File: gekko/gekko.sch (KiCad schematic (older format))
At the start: 83 parts, among them J10 Conn_01x02, J11 Conn_01x02, J3 Conn_01x05, J4 Conn_01x03, J6 Conn_01x02, Q5 IRLML6344TRPBFTR, SW1 SW_Push_Dual_x2, SW2 SW_DPDT_x2, U1 DRV8835, U12 sw_pch, U2 STM32F413CH6, U3 LED_FOTR, U4 LP5907_DBV, U5 ICM20648, U6 LED_FOTR, U7 LED_FOTR, U8 LED_FOTR, U9 RP124N334E-TR-FE, Y1 Crystal_GND23

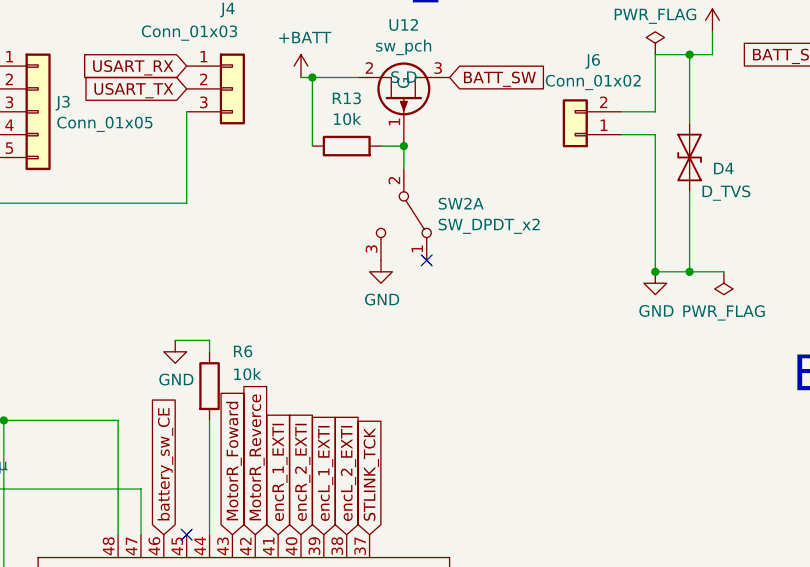
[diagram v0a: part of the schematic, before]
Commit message: betaGND
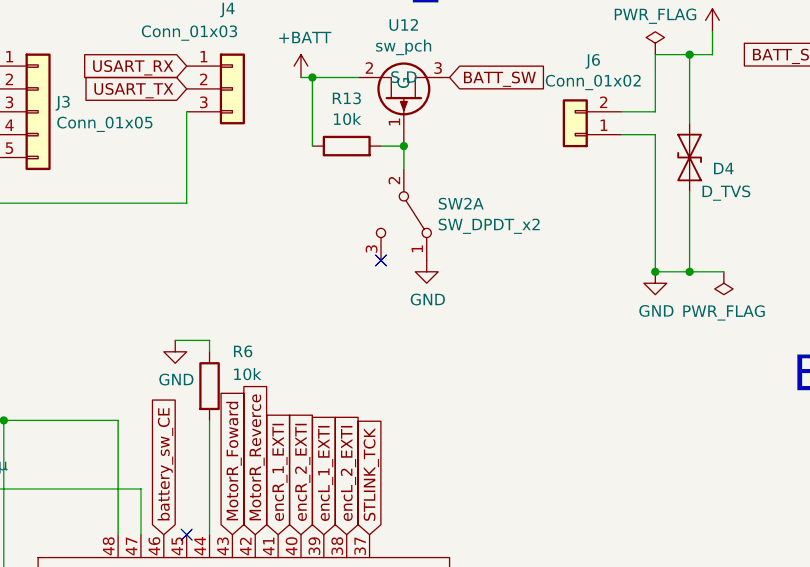
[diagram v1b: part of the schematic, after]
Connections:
- net GND: now also SW2.1 (A); no longer SW2.3 (C)
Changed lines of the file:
@@
 L power:GND #PWR021
 U 1 1 5EA1CF16
-P 6650 2000
-F 0 "#PWR021" H 6650 1750 50  0001 C CNN
-F 1 "GND" H 6655 1827 50  0000 C CNN
-F 2 "" H 6650 2000 50  0001 C CNN
-F 3 "" H 6650 2000 50  0001 C CNN
-	1    6650 2000
+P 6850 2000
+F 0 "#PWR021" H 6850 1750 50  0001 C CNN
+F 1 "GND" H 6855 1827 50  0000 C CNN
+F 2 "" H 6850 2000 50  0001 C CNN
+F 3 "" H 6850 2000 50  0001 C CNN
+	1    6850 2000
 	1    0    0    -1
 $EndComp
@@
 Wire Wire Line
 	4800 7100 4800 7200
-NoConn ~ 6850 2000
+NoConn ~ 6650 2000
 Text GLabel 5800 1150 0    50   Input ~ 0
 USART_RX

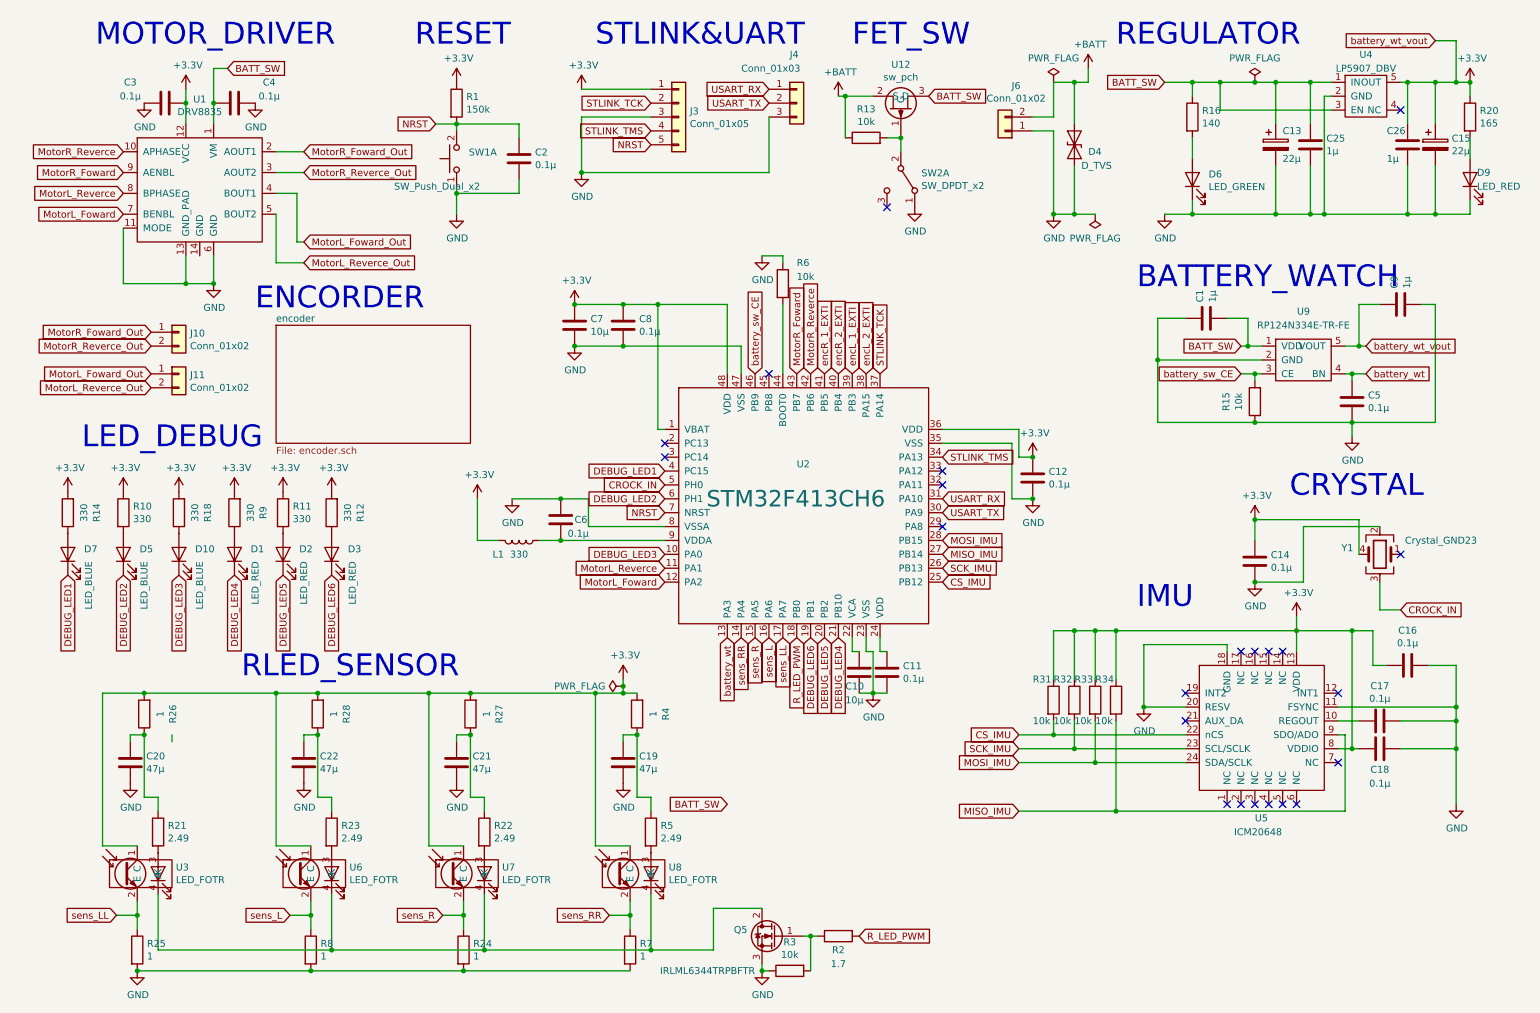
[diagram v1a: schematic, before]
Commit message: hattyu_v2
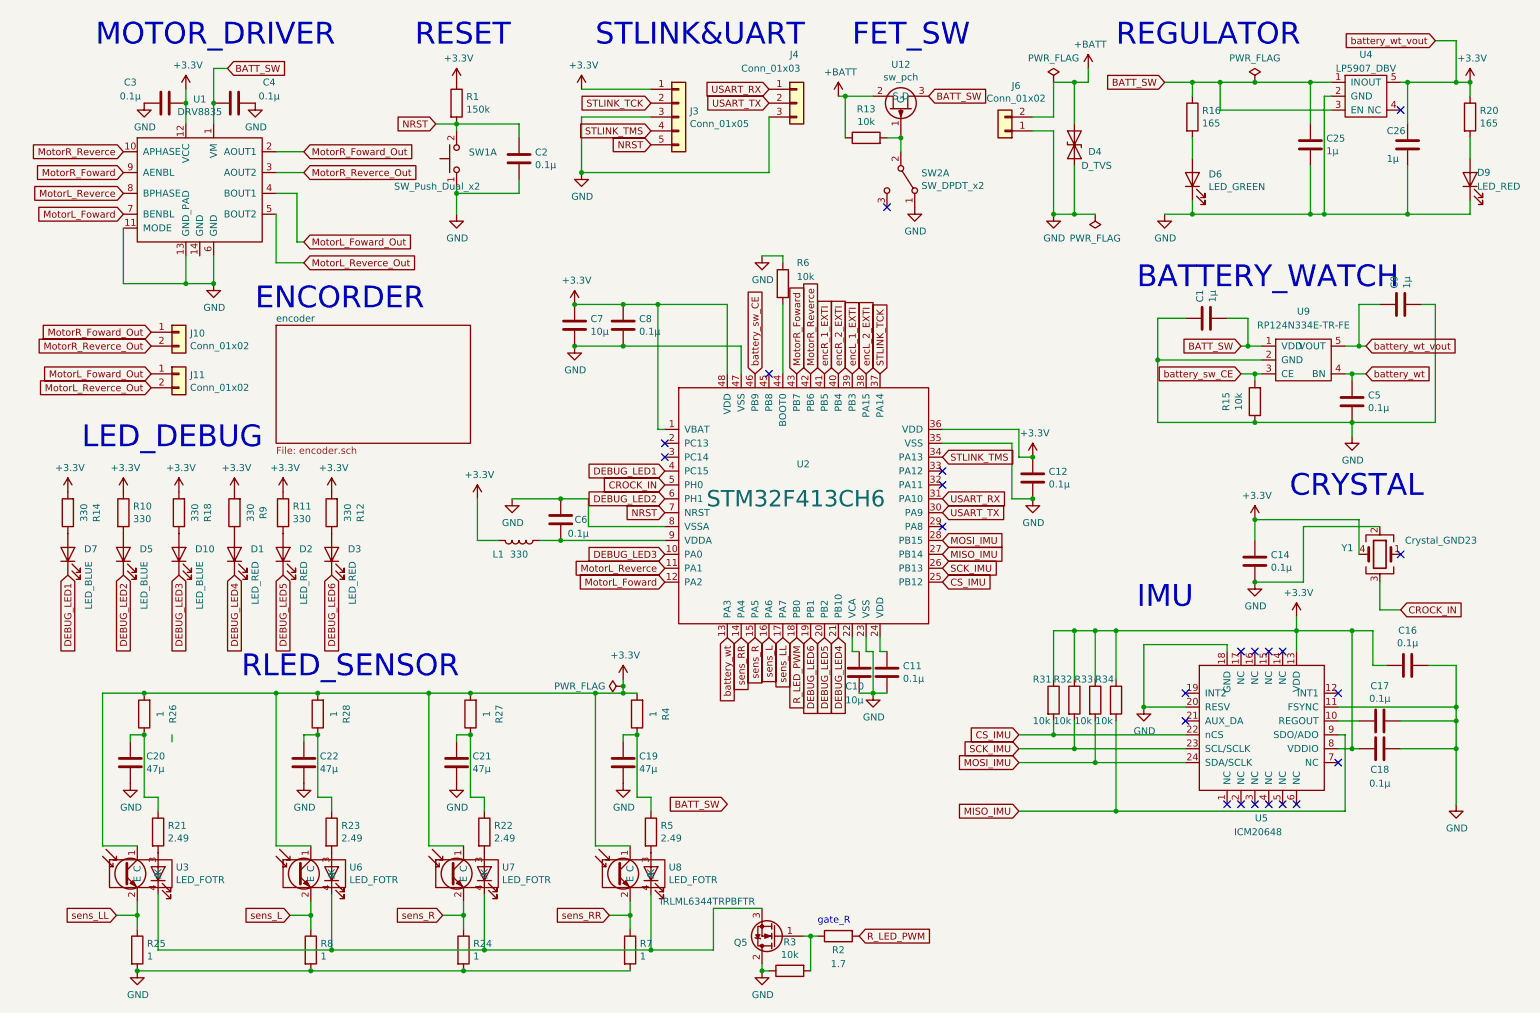
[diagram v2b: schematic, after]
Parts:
- removed C13, C15: 22μ, micro:6SVP22M, symbol gekko-rescue:CP-Device
- R16: value 140 -> 165
- U1: manf# (none) -> 296-30391-1-ND
- U2: manf# (none) -> 497-17018-ND
- U4: manf# (none) -> 296-38557-1-ND
- U5: manf# (none) -> 1428-1061-1-ND
- Y1: manf# (none) -> 535-11177-1-ND
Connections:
- net GND: now also Q5.2 (D); no longer Q5.3 (S)
- net at U3.4 (K), U6.4 (K), U7.4 (K)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: now also Q5.3 (S); no longer Q5.2 (D)
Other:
- note added: "gate_R\n\n"
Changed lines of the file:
@@
 F 3 "~" H 5850 7250 50  0001 C CNN
 	1    5850 7250
-	-1   0    0    -1
+	-1   0    0    1
 $EndComp
 Wire Wire Line
@@
 	7850 1100 7850 1350
 $Comp
-L gekko-rescue:CP-Device C13
-U 1 1 5E705C44
-P 9450 1550
-F 0 "C13" H 9500 1650 50  0000 L CNN
-F 1 "22μ" H 9500 1450 50  0000 L CNN
-F 2 "micro:6SVP22M" H 9488 1400 50  0001 C CNN
-F 3 "~" H 9450 1550 50  0001 C CNN
-	1    9450 1550
-	1    0    0    -1
-$EndComp
-Wire Wire Line
-	9450 1100 9450 1400
-Wire Wire Line
-	9450 2050 9450 1700
-$Comp
 L gekko-rescue:R-Device R16
 U 1 1 5E72594D
 P 8850 1350
 F 0 "R16" H 8920 1396 50  0000 L CNN
-F 1 "140" H 8920 1305 50  0000 L CNN
+F 1 "165" H 8920 1305 50  0000 L CNN
 F 2 "Resistor_SMD:R_0402_1005Metric" V 8780 1350 50  0001 C CNN
 F 3 "~" H 8850 1350 50  0001 C CNN
@@
 F 2 "micro:DRV8835DSSR" H 1700 1100 50  0001 C CNN
 F 3 "" H 1700 1100 50  0001 C CNN
+F 4 "296-30391-1-ND" H 1700 1450 50  0001 C CNN "manf#"
 	1    1700 1450
 	1    0    0    -1
@@
 F 2 "micro:STM32F411CEU6" H 6050 3200 50  0001 C CNN
 F 3 "" H 6050 3200 50  0001 C CNN
+F 4 "497-17018-ND" H 6050 3200 50  0001 C CNN "manf#"
 	1    6050 3200
 	1    0    0    -1
@@
 F 2 "micro:ICM20648" H 9350 3900 50  0001 C CNN
 F 3 "" H 9350 3900 50  0001 C CNN
+F 4 "1428-1061-1-ND" H 9350 5200 50  0001 C CNN "manf#"
 	1    9350 5200
 	1    0    0    -1
@@
 F 2 "micro:LP5907MFX-3.3&slash_NOPB" H 10100 1000 50  0001 C CNN
 F 3 "" H 10100 1000 50  0001 C CNN
+F 4 "296-38557-1-ND" H 10100 1000 50  0001 C CNN "manf#"
 	1    10100 1000
 	1    0    0    -1
@@
 NoConn ~ 10350 1300
 $Comp
-L gekko-rescue:CP-Device C15
-U 1 1 5DA4AB68
-P 10600 1550
-F 0 "C15" H 10718 1596 50  0000 L CNN
-F 1 "22μ" H 10718 1505 50  0000 L CNN
-F 2 "micro:6SVP22M" H 10638 1400 50  0001 C CNN
-F 3 "~" H 10600 1550 50  0001 C CNN
-	1    10600 1550
-	1    0    0    -1
-$EndComp
-Wire Wire Line
-	10600 1100 10600 1400
-Wire Wire Line
-	10600 1700 10600 2050
-$Comp
 L gekko-rescue:Crystal_GND23-Device Y1
 U 1 1 5DA8662B
@@
 F 2 "micro:crystal" H 10200 4500 50  0001 C CNN
 F 3 "~" H 10200 4500 50  0001 C CNN
+F 4 "535-11177-1-ND" H 10200 4500 50  0001 C CNN "manf#"
 	1    10200 4500
 	-1   0    0    -1
@@
 Wire Wire Line
 	10850 1950 10850 2050
-Wire Wire Line
-	10850 2050 10600 2050
 Text Notes 8450 4900 0    157  ~ 0
 IMU
@@
 Wire Wire Line
 	9700 1700 9700 2050
-Connection ~ 10600 1100
-Wire Wire Line
-	10600 1100 10750 1100
-Connection ~ 10600 2050
 Wire Wire Line
 	9800 2050 10400 2050
@@
 Connection ~ 10400 1100
 Wire Wire Line
-	10400 1100 10600 1100
-Wire Wire Line
 	10400 1700 10400 2050
 Connection ~ 10400 2050
-Wire Wire Line
-	10400 2050 10600 2050
 Wire Wire Line
 	6100 7250 6100 7500
@@
 Text GLabel 2450 2400 2    50   Input ~ 0
 MotorL_Reverce_Out
-Wire Wire Line
-	9300 1100 9450 1100
-Connection ~ 9450 1100
-Wire Wire Line
-	9450 1100 9700 1100
-Connection ~ 9450 2050
-Wire Wire Line
-	9450 2050 9700 2050
 Connection ~ 9700 1100
 Wire Wire Line
@@
 Wire Wire Line
 	8850 1100 9050 1100
-Wire Wire Line
-	8850 2050 9450 2050
 $Comp
 L gekko-rescue:GND-power #PWR029
@@
 Wire Wire Line
 	8300 5050 8300 5400
+Text Notes 6150 7250 0    50   ~ 0
+gate_R\n\n
+Wire Wire Line
+	8850 2050 9700 2050
+Wire Wire Line
+	9300 1100 9700 1100
+Wire Wire Line
+	10400 1100 10750 1100
+Wire Wire Line
+	10400 2050 10850 2050
 $EndSCHEMATC
